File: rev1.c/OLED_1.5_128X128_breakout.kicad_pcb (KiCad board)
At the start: 2 copper layers, 44 x 44 mm, 20 parts, among them P1 BREAKOUT, U1 FAN5331SX, U2 ER_OLED015_1C

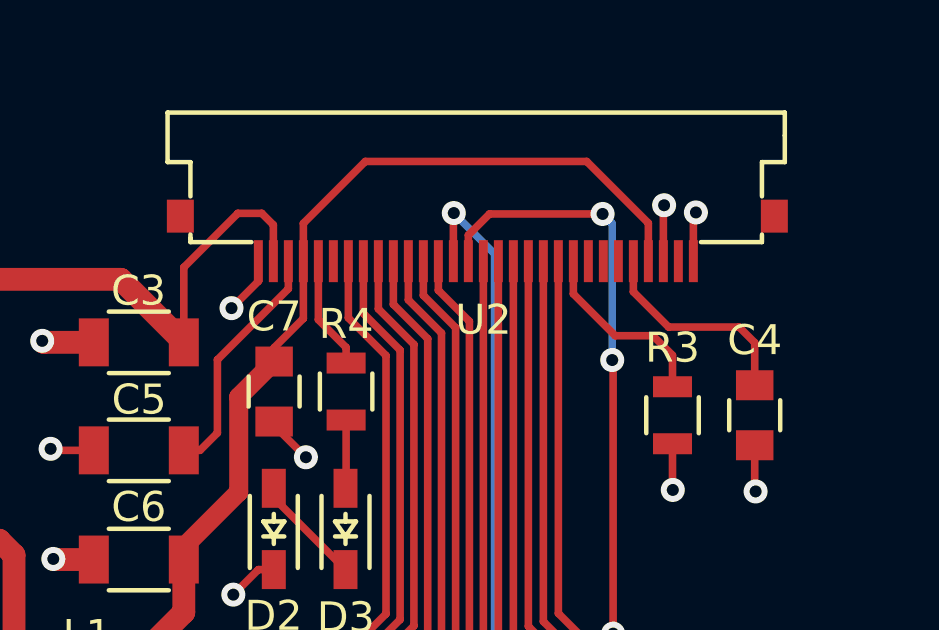
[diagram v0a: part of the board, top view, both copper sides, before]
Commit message: efficiency check and new gerbers
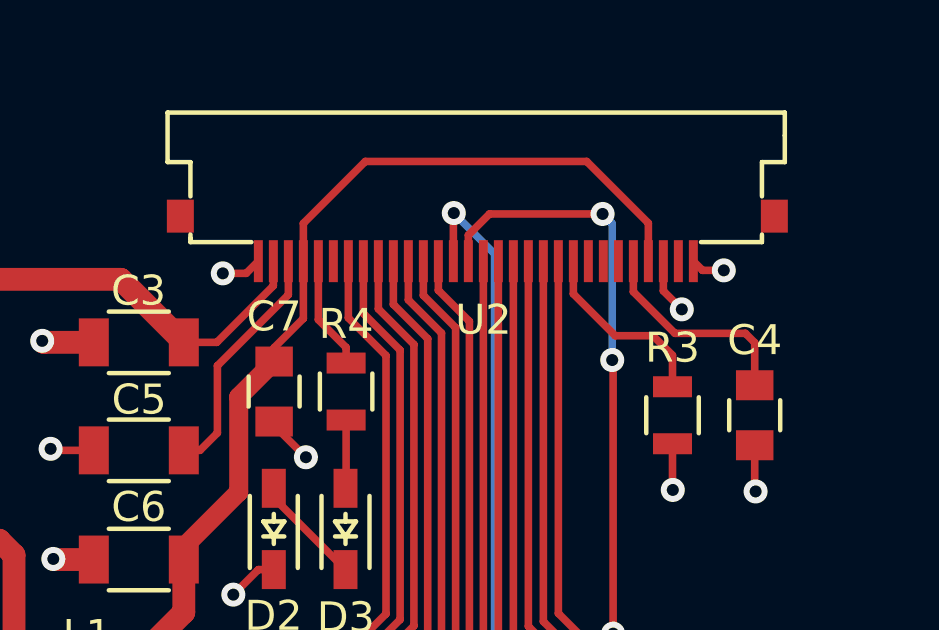
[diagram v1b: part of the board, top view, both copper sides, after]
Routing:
- net /+13V: track 41.0 -> 38.0 mm
- net GND: track 24.2 -> 23.1 mm
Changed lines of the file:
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@@
     (thickness 1.6)
     (drawings 27)
-    (tracks 202)
+    (tracks 200)
     (zones 0)
     (modules 20)
@@
   (page A4)
   (layers
-    (0 F.Cu signal hide)
+    (0 F.Cu signal)
     (31 B.Cu signal hide)
     (32 B.Adhes user)
@@
   (segment (start 54.75 85) (end 55.75 85) (width 0.762) (layer F.Cu) (net 1))
   (segment (start 54.3 89) (end 54.3 85.45) (width 0.762) (layer F.Cu) (net 1))
+  (via (at 80 60.1) (size 0.8) (drill 0.4) (layers F.Cu B.Cu) (net 2))
+  (segment (start 80 60.1) (end 79.291 60.1) (width 0.254) (layer F.Cu) (net 2))
+  (segment (start 79.291 60.1) (end 78.985 59.794) (width 0.254) (layer F.Cu) (net 2))
+  (via (at 63.3 60.2) (size 0.8) (drill 0.4) (layers F.Cu B.Cu) (net 2))
+  (segment (start 63.3 60.2) (end 64.079 60.2) (width 0.254) (layer F.Cu) (net 2))
+  (segment (start 64.079 60.2) (end 64.485 59.794) (width 0.254) (layer F.Cu) (net 2))
+  (segment (start 77.985 59.794) (end 77.985 60.785) (width 0.254) (layer F.Cu) (net 2))
+  (segment (start 77.985 60.785) (end 78.6 61.4) (width 0.254) (layer F.Cu) (net 2))
+  (via (at 78.6 61.4) (size 0.8) (drill 0.4) (layers F.Cu B.Cu) (net 2))
   (segment (start 65 70.075) (end 64.485 70.075) (width 0.254) (layer F.Cu) (net 2))
   (via (at 63.65 70.91) (size 0.8) (drill 0.4) (layers F.Cu B.Cu) (net 2))
   (segment (start 64.485 70.075) (end 63.65 70.91) (width 0.254) (layer F.Cu) (net 2))
-  (segment (start 78.985 59.794) (end 78.985 58.255) (width 0.254) (layer F.Cu) (net 2))
-  (via (at 79.07 58.17) (size 0.8) (drill 0.4) (layers F.Cu B.Cu) (net 2))
-  (segment (start 78.985 58.255) (end 79.07 58.17) (width 0.254) (layer F.Cu) (net 2))
-  (segment (start 77.985 59.794) (end 77.985 57.955) (width 0.254) (layer F.Cu) (net 2))
-  (via (at 78.01 57.93) (size 0.8) (drill 0.4) (layers F.Cu B.Cu) (net 2))
-  (segment (start 77.985 57.955) (end 78.01 57.93) (width 0.254) (layer F.Cu) (net 2))
   (segment (start 81.03 65.93) (end 81.03 67.44) (width 0.254) (layer F.Cu) (net 2))
   (segment (start 81.06 67.47) (end 81.08 67.47) (width 0.254) (layer B.Cu) (net 2))
@@
   (via (at 78.3 67.42) (size 0.8) (drill 0.4) (layers F.Cu B.Cu) (net 2))
   (segment (start 78.29 67.41) (end 78.3 67.42) (width 0.254) (layer F.Cu) (net 2))
-  (segment (start 64.485 59.794) (end 64.485 60.465) (width 0.254) (layer F.Cu) (net 2))
-  (segment (start 64.485 60.465) (end 63.59 61.36) (width 0.254) (layer F.Cu) (net 2))
-  (via (at 63.59 61.36) (size 0.8) (drill 0.4) (layers F.Cu B.Cu) (net 2))
   (segment (start 59 66.1) (end 57.61 66.1) (width 0.254) (layer F.Cu) (net 2))
   (via (at 57.56 66.05) (size 0.8) (drill 0.4) (layers F.Cu B.Cu) (net 2))
@@
   (segment (start 54.45 80.75) (end 54.4 80.8) (width 0.381) (layer F.Cu) (net 2))
   (via (at 54.4 80.8) (size 0.8) (drill 0.4) (layers F.Cu B.Cu) (net 2))
+  (segment (start 64.985 60.615) (end 63.1 62.5) (width 0.254) (layer F.Cu) (net 3))
+  (segment (start 63.1 62.5) (end 62 62.5) (width 0.254) (layer F.Cu) (net 3))
+  (segment (start 64.985 59.794) (end 64.985 60.615) (width 0.254) (layer F.Cu) (net 3))
   (segment (start 54.7 60.4) (end 59.9 60.4) (width 0.762) (layer F.Cu) (net 3))
   (segment (start 59.9 60.4) (end 62 62.5) (width 0.762) (layer F.Cu) (net 3))
   (segment (start 52 63.1) (end 54.7 60.4) (width 0.762) (layer F.Cu) (net 3))
   (segment (start 52 71.18) (end 52 63.1) (width 0.762) (layer F.Cu) (net 3))
-  (segment (start 63.8 58.2) (end 62 60) (width 0.254) (layer F.Cu) (net 3))
-  (segment (start 62 60) (end 62 62.5) (width 0.254) (layer F.Cu) (net 3))
-  (segment (start 64.6 58.2) (end 63.8 58.2) (width 0.254) (layer F.Cu) (net 3))
-  (segment (start 64.985 58.585) (end 64.6 58.2) (width 0.254) (layer F.Cu) (net 3))
-  (segment (start 64.985 59.794) (end 64.985 58.585) (width 0.254) (layer F.Cu) (net 3))
   (segment (start 52 79.05) (end 52 71.18) (width 0.762) (layer F.Cu) (net 3))
   (segment (start 54.59 72.365) (end 53.185 72.365) (width 0.762) (layer F.Cu) (net 3))
@@
   (segment (start 55.65 81.7) (end 52.75 81.7) (width 0.381) (layer F.Cu) (net 4))
   (segment (start 52.75 81.7) (end 52 80.95) (width 0.381) (layer F.Cu) (net 4))
-  (segment (start 80.51 61.99) (end 81.03 62.51) (width 0.254) (layer F.Cu) (net 5))
+  (segment (start 76.985 59.794) (end 76.985 60.815) (width 0.254) (layer F.Cu) (net 5))
+  (segment (start 76.985 60.815) (end 78.37 62.2) (width 0.254) (layer F.Cu) (net 5))
+  (segment (start 78.37 62.2) (end 80.72 62.2) (width 0.254) (layer F.Cu) (net 5))
+  (segment (start 80.72 62.2) (end 81.03 62.51) (width 0.254) (layer F.Cu) (net 5))
   (segment (start 81.03 62.51) (end 81.03 63.93) (width 0.254) (layer F.Cu) (net 5))
-  (segment (start 78.16 61.99) (end 80.51 61.99) (width 0.254) (layer F.Cu) (net 5))
-  (segment (start 76.985 60.815) (end 78.16 61.99) (width 0.254) (layer F.Cu) (net 5))
-  (segment (start 76.985 59.794) (end 76.985 60.815) (width 0.254) (layer F.Cu) (net 5))
+  (segment (start 65.485 59.794) (end 65.485 60.915) (width 0.254) (layer F.Cu) (net 6))
+  (segment (start 65.485 60.915) (end 63.12 63.28) (width 0.254) (layer F.Cu) (net 6))
+  (segment (start 63.12 63.28) (end 63.12 65.52) (width 0.254) (layer F.Cu) (net 6))
   (segment (start 63.12 65.52) (end 62.54 66.1) (width 0.254) (layer F.Cu) (net 6))
   (segment (start 62.54 66.1) (end 62 66.1) (width 0.254) (layer F.Cu) (net 6))
-  (segment (start 63.12 63.08) (end 63.12 65.52) (width 0.254) (layer F.Cu) (net 6))
-  (segment (start 65.485 60.715) (end 63.12 63.08) (width 0.254) (layer F.Cu) (net 6))
-  (segment (start 65.485 59.794) (end 65.485 60.715) (width 0.254) (layer F.Cu) (net 6))
   (segment (start 55.65 78.77) (end 57.71 76.71) (width 0.762) (layer F.Cu) (net 7))
   (segment (start 57.71 76.71) (end 58.79 76.71) (width 0.762) (layer F.Cu) (net 7))
